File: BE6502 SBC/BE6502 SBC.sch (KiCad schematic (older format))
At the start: 53 parts, among them J1 Expansion, J3 BARREL_JACK, M1 Mounting, M2 Mounting, M3 Mounting, M4 Mounting, SW1 RESET, SW2 RESET, SW3 RESET, SW4 RESET, SW5 RESET, SW6 RESET, U1 W65C02, U2 HM62256BLP-7, U3 28C256, U4 WD65C22, U5 74HC00, U6 RC1602A, X1 1MHz

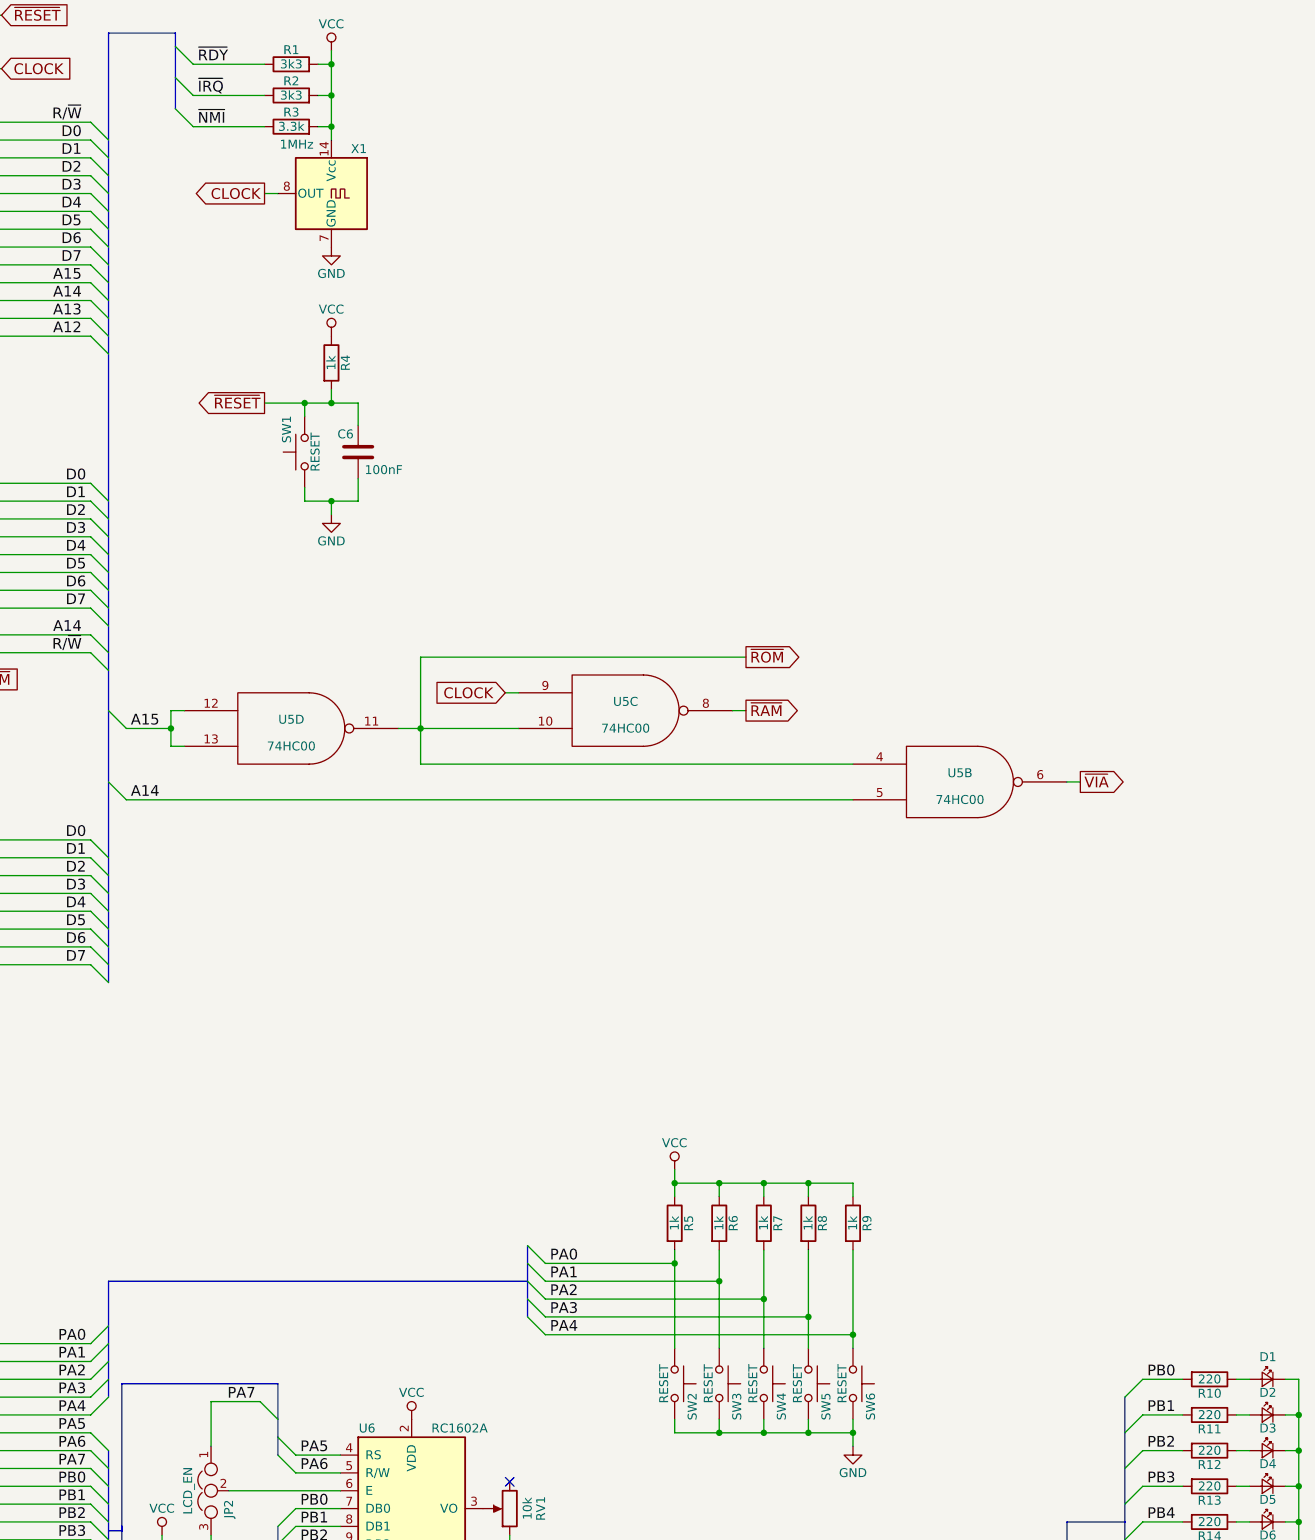
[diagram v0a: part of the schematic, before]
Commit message: Component placement
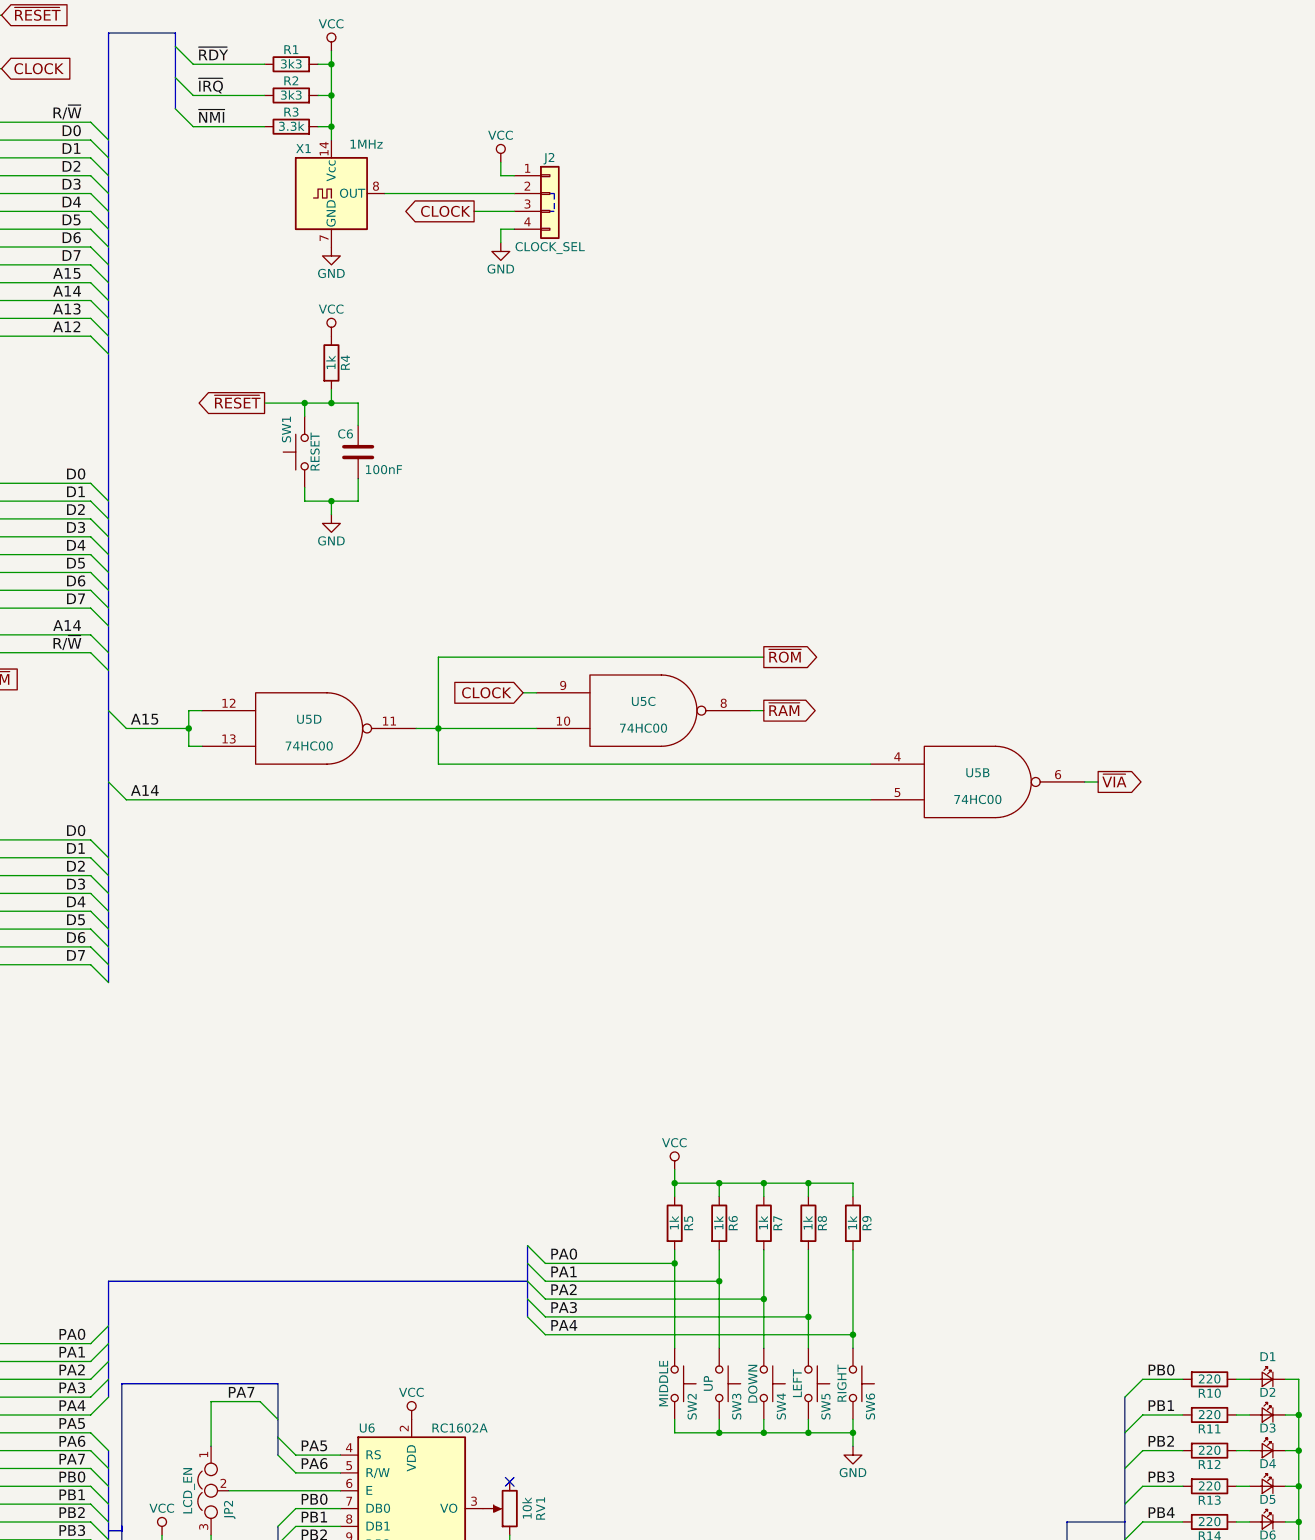
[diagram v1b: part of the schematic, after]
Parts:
- added J2: CLOCK_SEL, Pin_Headers:Pin_Header_Angled_1x04_Pitch2.54mm, symbol Conn_01x04
- D1, D2, D3, D4, D5, D6, D7, D8: footprint (none) -> LEDs:LED_D5.0mm
- J1: footprint (none) -> Pin_Headers:Pin_Header_Angled_1x39_Pitch2.54mm
- JP1: footprint (none) -> Pin_Headers:Pin_Header_Straight_1x02_Pitch2.54mm
- JP2: footprint (none) -> Pin_Headers:Pin_Header_Straight_1x03_Pitch2.54mm
- RV1: footprint (none) -> Potentiometers:Potentiometer_Trimmer_Bourns_3296W
- SW1: footprint (none) -> Buttons_Switches_THT:SW_PUSH_6mm
- SW2: value RESET -> MIDDLE; footprint (none) -> Buttons_Switches_THT:SW_PUSH_6mm
- SW3: value RESET -> UP; footprint (none) -> Buttons_Switches_THT:SW_PUSH_6mm
- SW4: value RESET -> DOWN; footprint (none) -> Buttons_Switches_THT:SW_PUSH_6mm
- SW5: value RESET -> LEFT; footprint (none) -> Buttons_Switches_THT:SW_PUSH_6mm
- SW6: value RESET -> RIGHT; footprint (none) -> Buttons_Switches_THT:SW_PUSH_6mm
- U1, U4: footprint (none) -> Housings_DIP:DIP-40_W15.24mm_Socket_LongPads
- U2, U3: footprint Housings_DIP:DIP-28_W15.24mm_Socket -> Housings_DIP:DIP-28_W15.24mm_Socket_LongPads
- U5: footprint (none) -> Housings_DIP:DIP-14_W7.62mm_Socket_LongPads
- U6: footprint Displays:RC1602A -> Displays:WC1602A
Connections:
- net CLOCK: now also J2.3 (Pin_3); no longer X1.8 (OUT)
- net GND: now also J2.4 (Pin_4)
- net VCC: now also J2.1 (Pin_1)
- new net: J2.2 (Pin_2), X1.8 (OUT)
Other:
- moved on the sheet: U5B, U5C, U5D, X1

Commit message: Layout done
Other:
- moved on the sheet: U5B
